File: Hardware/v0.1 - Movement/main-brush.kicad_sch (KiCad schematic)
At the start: 3 parts, among them J4 Brush Motor Main, Q4 IRF540N

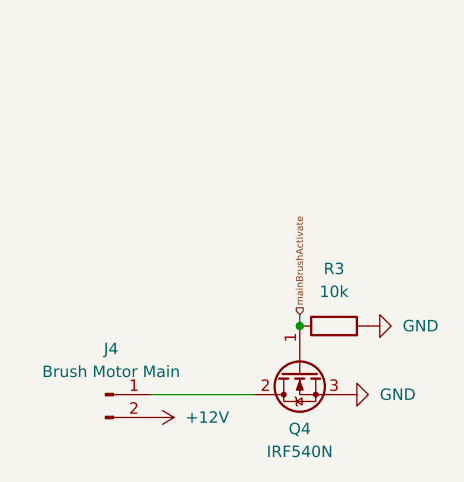
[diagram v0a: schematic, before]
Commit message: added session 17
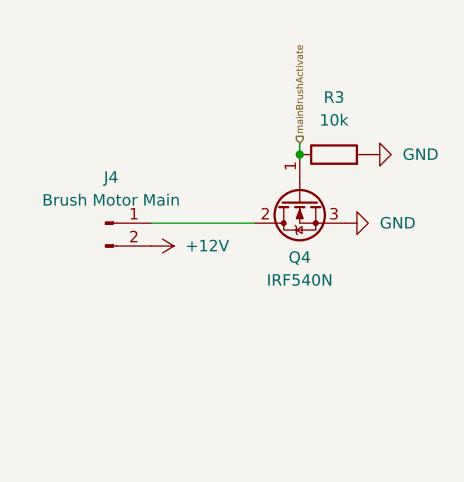
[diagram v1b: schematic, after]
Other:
- moved on the sheet: R3
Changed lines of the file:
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@@
 	)
 	(junction
-		(at 146.05 109.22)
+		(at 146.05 90.17)
 		(diameter 0)
 		(color 0 0 0 0)
@@
 	(wire
 		(pts
-			(xy 146.05 107.95) (xy 146.05 109.22)
+			(xy 146.05 88.9) (xy 146.05 90.17)
 		)
 		(stroke
@@
 	(wire
 		(pts
-			(xy 129.54 116.84) (xy 140.97 116.84)
+			(xy 129.54 97.79) (xy 140.97 97.79)
 		)
 		(stroke
@@
 	(hierarchical_label "mainBrushActivate"
 		(shape input)
-		(at 146.05 107.95 90)
+		(at 146.05 88.9 90)
 		(fields_autoplaced yes)
 		(effects
@@
 	(symbol
 		(lib_id "power:+12V")
-		(at 129.54 119.38 270)
+		(at 129.54 100.33 270)
 		(unit 1)
 		(exclude_from_sim no)
@@
 		(fields_autoplaced yes)
 		(property "Reference" "#PWR06"
-			(at 125.73 119.38 0)
+			(at 125.73 100.33 0)
 			(effects
 				(font
@@
 		)
 		(property "Value" "+12V"
-			(at 133.35 119.3799 90)
+			(at 133.35 100.3299 90)
 			(effects
 				(font
@@
 		)
 		(property "Footprint" ""
-			(at 129.54 119.38 0)
+			(at 129.54 100.33 0)
 			(effects
 				(font
@@
 		)
 		(property "Datasheet" ""
-			(at 129.54 119.38 0)
+			(at 129.54 100.33 0)
 			(effects
 				(font
@@
 		)
 		(property "Description" "Power symbol creates a global label with name \"+12V\""
-			(at 129.54 119.38 0)
+			(at 129.54 100.33 0)
 			(effects
 				(font
@@
 	(symbol
 		(lib_id "Device:R")
-		(at 149.86 109.22 90)
+		(at 149.86 90.17 90)
 		(unit 1)
 		(exclude_from_sim no)
@@
 		(fields_autoplaced yes)
 		(property "Reference" "R3"
-			(at 149.86 102.87 90)
+			(at 149.86 83.82 90)
 			(effects
 				(font
@@
 		)
 		(property "Value" "10k"
-			(at 149.86 105.41 90)
+			(at 149.86 86.36 90)
 			(effects
 				(font
@@
 		)
 		(property "Footprint" "Resistor_THT:R_Axial_DIN0207_L6.3mm_D2.5mm_P10.16mm_Horizontal"
-			(at 149.86 110.998 90)
+			(at 149.86 91.948 90)
 			(effects
 				(font
@@
 		)
 		(property "Datasheet" "~"
-			(at 149.86 109.22 0)
+			(at 149.86 90.17 0)
 			(effects
 				(font
@@
 		)
 		(property "Description" "Resistor"
-			(at 149.86 109.22 0)
+			(at 149.86 90.17 0)
 			(effects
 				(font
@@
 	)
 	(symbol
+		(lib_id "Connector:Conn_01x02_Pin")
+		(at 124.46 97.79 0)
+		(unit 1)
+		(exclude_from_sim no)
+		(in_bom yes)
+		(on_board yes)
+		(dnp no)
+		(fields_autoplaced yes)
+		(property "Reference" "J4"
+			(at 125.095 92.71 0)
+			(effects
+				(font
+					(size 1.27 1.27)
+				)
+			)
+		)
+		(property "Value" "Brush Motor Main"
+			(at 125.095 95.25 0)
+			(effects
+				(font
+					(size 1.27 1.27)
+				)
+			)
+		)
+		(property "Footprint" "Connector_JST:JST_PH_B2B-PH-K_1x02_P2.00mm_Vertical"
+			(at 124.46 97.79 0)
+			(effects
+				(font
+					(size 1.27 1.27)
+				)
+				(hide yes)
+			)
+		)
+		(property "Datasheet" "~"
+			(at 124.46 97.79 0)
+			(effects
+				(font
+					(size 1.27 1.27)
+				)
+				(hide yes)
+			)
+		)
+		(property "Description" "Generic connector, single row, 01x02, script generated"
+			(at 124.46 97.79 0)
+			(effects
+				(font
+					(size 1.27 1.27)
+				)
+				(hide yes)
+			)
+		)
+		(pin "2"
+		)
+		(pin "1"
+		)
+		(instances
+			(project "openVac-v0.1"
+				(path "/51937001-9622-40ac-b790-90fb4ff028f7/ac46296d-1959-48c3-a456-a22caced9bcf"
+					(reference "J4")
+					(unit 1)
+				)
+			)
+		)
+	)
+	(symbol
 		(lib_id "power:GND")
-		(at 151.13 116.84 90)
+		(at 151.13 97.79 90)
 		(unit 1)
 		(exclude_from_sim no)
@@
 		(fields_autoplaced yes)
 		(property "Reference" "#PWR08"
-			(at 157.48 116.84 0)
+			(at 157.48 97.79 0)
 			(effects
 				(font
@@
 		)
 		(property "Value" "GND"
-			(at 154.94 116.8399 90)
+			(at 154.94 97.7899 90)
 			(effects
 				(font
@@
 		)
 		(property "Footprint" ""
-			(at 151.13 116.84 0)
+			(at 151.13 97.79 0)
 			(effects
 				(font
@@
 		)
 		(property "Datasheet" ""
-			(at 151.13 116.84 0)
+			(at 151.13 97.79 0)
 			(effects
 				(font
@@
 		)
 		(property "Description" "Power symbol creates a global label with name \"GND\" , ground"
-			(at 151.13 116.84 0)
+			(at 151.13 97.79 0)
 			(effects
 				(font
@@
 	(symbol
 		(lib_id "Transistor_FET:IRF540N")
-		(at 146.05 114.3 90)
+		(at 146.05 95.25 90)
 		(mirror x)
 		(unit 1)
@@
 		(dnp no)
 		(property "Reference" "Q4"
-			(at 146.05 120.65 90)
+			(at 146.05 101.6 90)
 			(effects
 				(font
@@
 		)
 		(property "Value" "IRF540N"
-			(at 146.05 123.19 90)
+			(at 146.05 104.14 90)
 			(effects
 				(font
@@
 		)
 		(property "Footprint" "Package_TO_SOT_THT:TO-220-3_Vertical"
-			(at 147.955 119.38 0)
+			(at 147.955 100.33 0)
 			(effects
 				(font
@@
 		)
 		(property "Datasheet" "http://www.irf.com/product-info/datasheets/data/irf540n.pdf"
-			(at 149.86 119.38 0)
+			(at 149.86 100.33 0)
 			(effects
 				(font
@@
 		)
 		(property "Description" "33A Id, 100V Vds, HEXFET N-Channel MOSFET, TO-220"
-			(at 146.05 114.3 0)
+			(at 146.05 95.25 0)
 			(effects
 				(font
@@
 	)
 	(symbol
-		(lib_id "Connector:Conn_01x02_Pin")
-		(at 124.46 116.84 0)
-		(unit 1)
-		(exclude_from_sim no)
-		(in_bom yes)
-		(on_board yes)
-		(dnp no)
-		(fields_autoplaced yes)
-		(property "Reference" "J4"
-			(at 125.095 111.76 0)
-			(effects
-				(font
-					(size 1.27 1.27)
-				)
-			)
-		)
-		(property "Value" "Brush Motor Main"
-			(at 125.095 114.3 0)
-			(effects
-				(font
-					(size 1.27 1.27)
-				)
-			)
-		)
-		(property "Footprint" "Connector_JST:JST_PH_B2B-PH-K_1x02_P2.00mm_Vertical"
-			(at 124.46 116.84 0)
-			(effects
-				(font
-					(size 1.27 1.27)
-				)
-				(hide yes)
-			)
-		)
-		(property "Datasheet" "~"
-			(at 124.46 116.84 0)
-			(effects
-				(font
-					(size 1.27 1.27)
-				)
-				(hide yes)
-			)
-		)
-		(property "Description" "Generic connector, single row, 01x02, script generated"
-			(at 124.46 116.84 0)
-			(effects
-				(font
-					(size 1.27 1.27)
-				)
-				(hide yes)
-			)
-		)
-		(pin "2"
-		)
-		(pin "1"
-		)
-		(instances
-			(project "openVac-v0.1"
-				(path "/51937001-9622-40ac-b790-90fb4ff028f7/ac46296d-1959-48c3-a456-a22caced9bcf"
-					(reference "J4")
-					(unit 1)
-				)
-			)
-		)
-	)
-	(symbol
 		(lib_id "power:GND")
-		(at 153.67 109.22 90)
+		(at 153.67 90.17 90)
 		(unit 1)
 		(exclude_from_sim no)
@@
 		(fields_autoplaced yes)
 		(property "Reference" "#PWR05"
-			(at 160.02 109.22 0)
+			(at 160.02 90.17 0)
 			(effects
 				(font
@@
 		)
 		(property "Value" "GND"
-			(at 157.48 109.2199 90)
+			(at 157.48 90.1699 90)
 			(effects
 				(font
@@
 		)
 		(property "Footprint" ""
-			(at 153.67 109.22 0)
+			(at 153.67 90.17 0)
 			(effects
 				(font
@@
 		)
 		(property "Datasheet" ""
-			(at 153.67 109.22 0)
+			(at 153.67 90.17 0)
 			(effects
 				(font
@@
 		)
 		(property "Description" "Power symbol creates a global label with name \"GND\" , ground"
-			(at 153.67 109.22 0)
-			(effects
-				(font
+			(at 153.67 90.17 0)
+			(effects
+				(font
